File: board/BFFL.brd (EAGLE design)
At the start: 51 x 25.4 mm, 25 parts, among them IC1 LM317MSTT3, Q1 FDS5680, U1 ATTINY84-20SSU, X1 MKDSN1,5/2-5,08, X2 22-23-2041, X3 22-23-2031, X4 22-23-2071

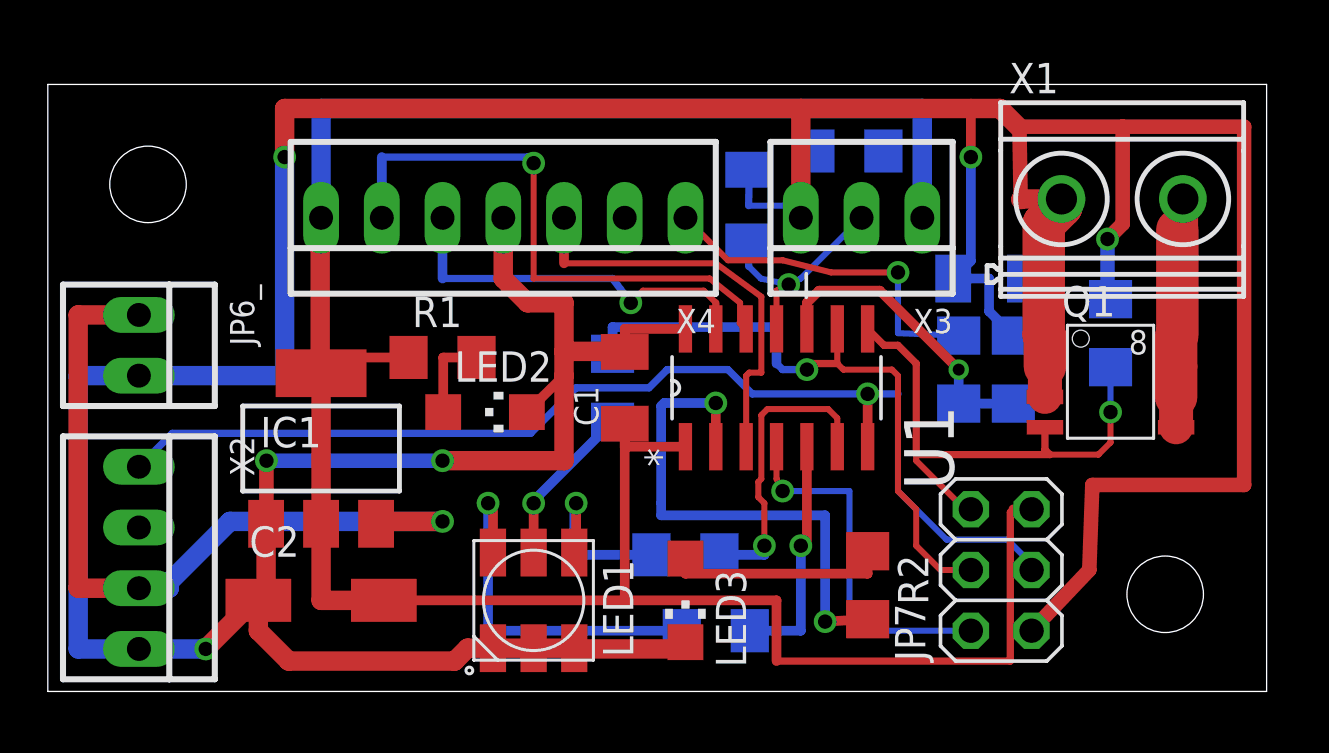
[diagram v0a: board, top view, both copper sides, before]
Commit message: Update board
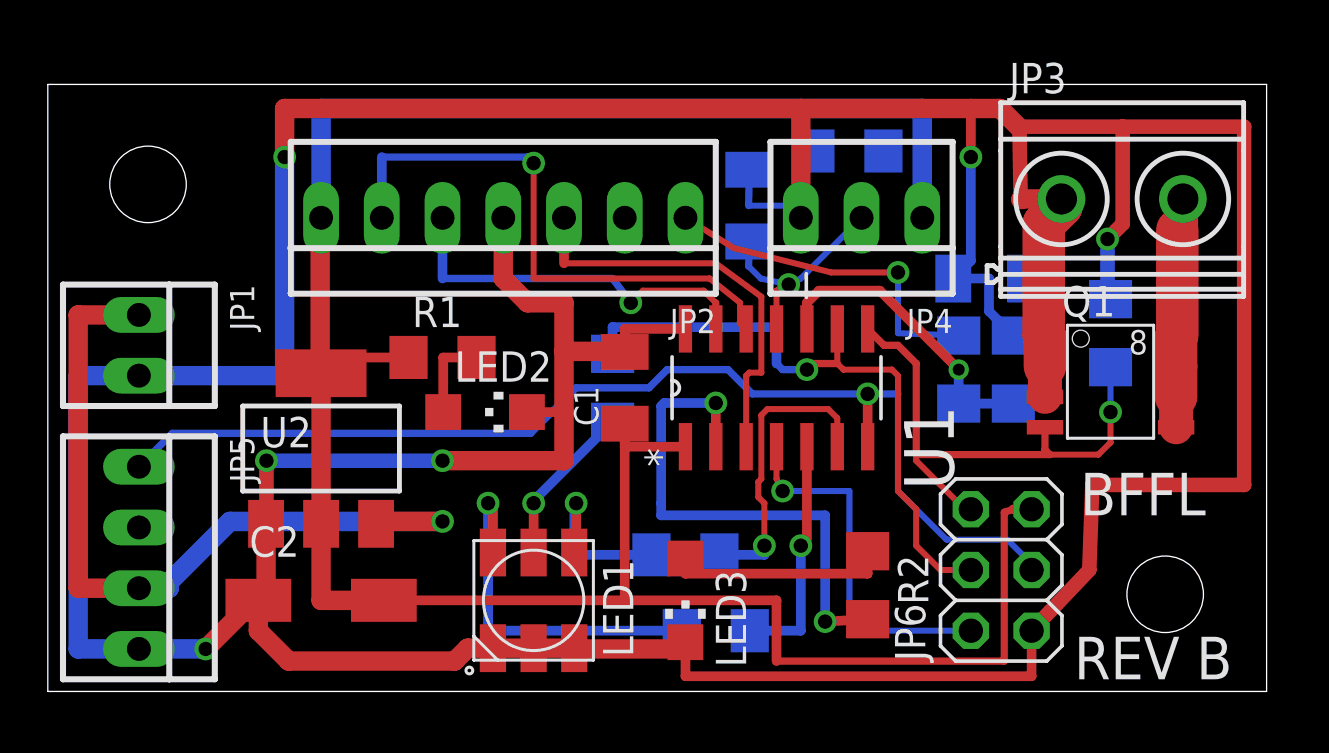
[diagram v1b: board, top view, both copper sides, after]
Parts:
- renumbered IC1 to U2, JP6_ to JP1, JP7 to JP6, X1 to JP3, X2 to JP5, X3 to JP4, X4 to JP2
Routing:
- net N$13: track 212.6 -> 229.2 mm
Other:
- board text added: "BFFL"
- board text added: "REV B"
